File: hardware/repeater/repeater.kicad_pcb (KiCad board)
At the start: 2 copper layers, 25.5 x 42 mm, 50 parts, among them J1 Screw_Terminal_01x06, J2 Conn_01x08, J3 Screw_Terminal_01x06, U1 TJA1051T-3, U2 74LVC1G00, U3 74LVC2G74, U6 TJA1051T-3, U8 TD1465

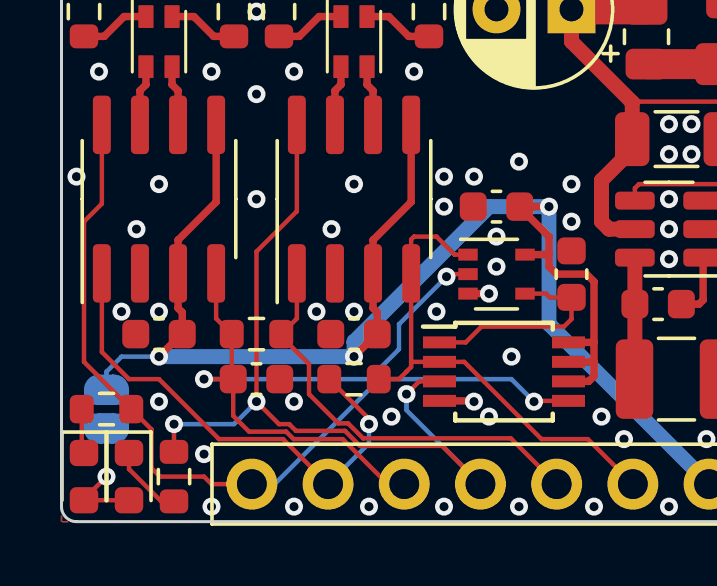
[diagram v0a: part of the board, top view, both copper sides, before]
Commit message: night light ready
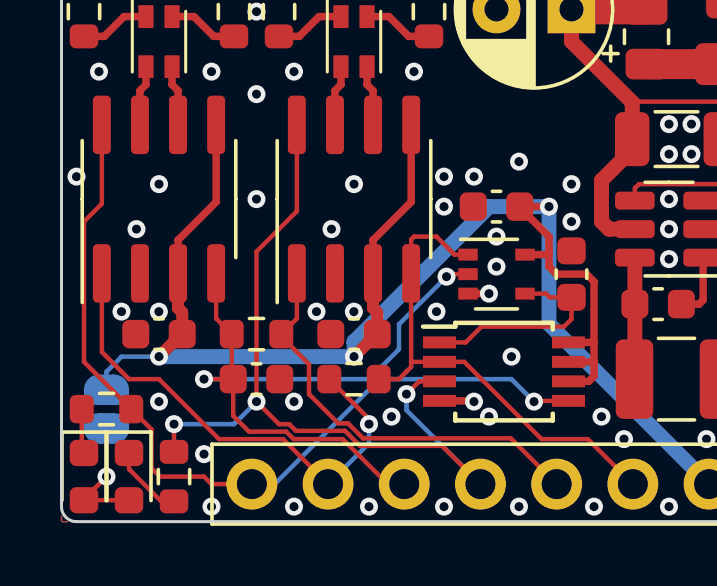
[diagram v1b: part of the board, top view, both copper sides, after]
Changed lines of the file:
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@@
   (via (at 122 78.75) (size 0.6) (drill 0.3) (layers "F.Cu" "B.Cu") (free) (net 1))
   (via (at 117 87.75) (size 0.6) (drill 0.3) (layers "F.Cu" "B.Cu") (free) (net 1))
-  (via (at 122 83) (size 0.6) (drill 0.3) (layers "F.Cu" "B.Cu") (free) (net 1))
+  (via (at 121.995896 83.000743) (size 0.6) (drill 0.3) (layers "F.Cu" "B.Cu") (free) (net 1))
   (via (at 123.25 86.5) (size 0.6) (drill 0.3) (layers "F.Cu" "B.Cu") (free) (net 1))
   (via (at 120.75 83) (size 0.6) (drill 0.3) (layers "F.Cu" "B.Cu") (free) (net 1))
@@
   (via (at 113.5 61) (size 0.6) (drill 0.3) (layers "F.Cu" "B.Cu") (free) (net 1))
   (via (at 132.5 80.25) (size 0.6) (drill 0.3) (layers "F.Cu" "B.Cu") (free) (net 1))
-  (via (at 115.5 83) (size 0.6) (drill 0.3) (layers "F.Cu" "B.Cu") (free) (net 1))
+  (via (at 115.495896 83.000743) (size 0.6) (drill 0.3) (layers "F.Cu" "B.Cu") (free) (net 1))
   (via (at 125 79.5) (size 0.6) (drill 0.3) (layers "F.Cu" "B.Cu") (free) (net 1))
   (via (at 132.5 81.25) (size 0.6) (drill 0.3) (layers "F.Cu" "B.Cu") (free) (net 1))
@@
   (segment (start 122.635 81.725) (end 122.635 80.615) (width 0.25) (layer "F.Cu") (net 21))
   (segment (start 122.775 83.75) (end 122.75 83.75) (width 0.25) (layer "F.Cu") (net 21))
-  (segment (start 122.635 81.725) (end 122.635 82.885) (width 0.25) (layer "F.Cu") (net 21))
-  (segment (start 122.75 83.75) (end 122 84.5) (width 0.25) (layer "F.Cu") (net 21))
+  (segment (start 122.635 81.725) (end 122.635 82.885) (width 0.4) (layer "F.Cu") (net 21))
+  (segment (start 122.75 83.75) (end 122 84.5) (width 0.4) (layer "F.Cu") (net 21))
   (segment (start 135.25 85.5) (end 135.95 86.2) (width 0.25) (layer "F.Cu") (net 21))
   (segment (start 134.149999 85.25) (end 134.15 85.9) (width 0.5) (layer "F.Cu") (net 21))
@@
   (segment (start 129.15 85.325) (end 129.825 85.325) (width 0.25) (layer "F.Cu") (net 21))
   (segment (start 116.135 80.615) (end 117.405 79.345) (width 0.25) (layer "F.Cu") (net 21))
-  (segment (start 116.275 83.025) (end 116.275 83.75) (width 0.25) (layer "F.Cu") (net 21))
+  (segment (start 116.275 83.025) (end 116.275 83.75) (width 0.4) (layer "F.Cu") (net 21))
   (segment (start 136.25 86.335) (end 133.835 88.75) (width 0.5) (layer "F.Cu") (net 21))
   (segment (start 117.405 79.345) (end 117.405 76.775) (width 0.25) (layer "F.Cu") (net 21))
-  (segment (start 122.635 82.885) (end 122.775 83.025) (width 0.25) (layer "F.Cu") (net 21))
-  (segment (start 122.775 83.025) (end 122.775 83.75) (width 0.25) (layer "F.Cu") (net 21))
+  (segment (start 122.635 82.885) (end 122.775 83.025) (width 0.4) (layer "F.Cu") (net 21))
+  (segment (start 122.775 83.025) (end 122.775 83.75) (width 0.4) (layer "F.Cu") (net 21))
   (segment (start 127.525 79.5) (end 128.5 79.5) (width 0.25) (layer "F.Cu") (net 21))
   (segment (start 135.95 86.2) (end 136.25 86.2) (width 0.25) (layer "F.Cu") (net 21))
-  (segment (start 116.25 83.75) (end 115.5 84.5) (width 0.25) (layer "F.Cu") (net 21))
+  (segment (start 116.25 83.75) (end 115.5 84.5) (width 0.4) (layer "F.Cu") (net 21))
   (segment (start 136.25 86.2) (end 136.25 86.335) (width 0.5) (layer "F.Cu") (net 21))
-  (segment (start 116.135 82.885) (end 116.275 83.025) (width 0.25) (layer "F.Cu") (net 21))
+  (segment (start 116.135 82.885) (end 116.275 83.025) (width 0.4) (layer "F.Cu") (net 21))
   (segment (start 128.75 81.75) (end 128.5 81.5) (width 0.25) (layer "F.Cu") (net 21))
   (segment (start 123.905 79.345) (end 123.905 76.775) (width 0.25) (layer "F.Cu") (net 21))
@@
   (segment (start 127.7 81.1) (end 128.5 81.1) (width 0.25) (layer "F.Cu") (net 21))
   (segment (start 122.635 80.615) (end 123.905 79.345) (width 0.25) (layer "F.Cu") (net 21))
-  (segment (start 116.135 81.725) (end 116.135 82.885) (width 0.25) (layer "F.Cu") (net 21))
+  (segment (start 116.135 81.725) (end 116.135 82.885) (width 0.4) (layer "F.Cu") (net 21))
   (segment (start 128.5 81.5) (end 128.5 81) (width 0.25) (layer "F.Cu") (net 21))
   (segment (start 129.825 85.325) (end 130 85.15) (width 0.25) (layer "F.Cu") (net 21))
